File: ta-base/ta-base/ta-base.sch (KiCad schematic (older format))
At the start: 15 parts, among them J1 PinSocket_16_base, J2 PinSocket_4_base, J3 PinSocket_5_base, J4 PinSocket_4_base, J5 PinSocket_5_base, J6 PinSocket_16_base, P1 Gnd_Screws, P2 Gnd_standoffs, SW1 SW_SPDT, SW2 SW_SPDT, U1 BSB008NE2LXXUMA1, U2 burn_wire

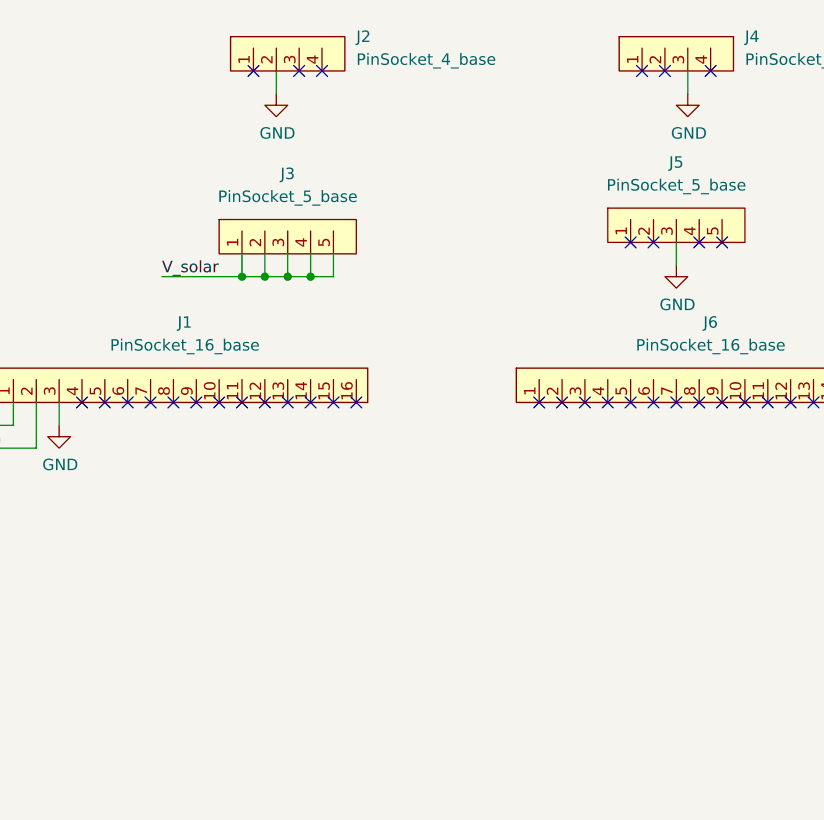
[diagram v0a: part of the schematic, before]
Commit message: finalized place and route
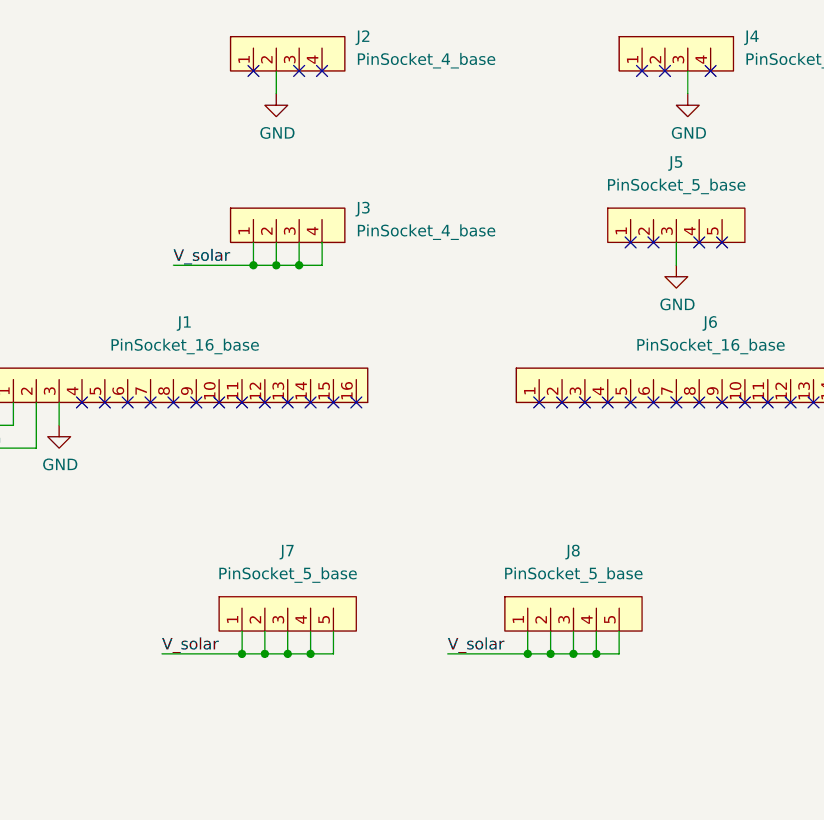
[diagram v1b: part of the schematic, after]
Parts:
- removed J3: PinSocket_5_base, symbol ta-base:PinSocket_5_base
- added J3: PinSocket_4_base, ta-base:PinSocket_1x4_TartanArtibeus_base_cpy, symbol ta-base:PinSocket_4_base
- added J7, J8: PinSocket_5_base, ta-base:solar_internal, symbol ta-base:PinSocket_5_base
- J4: footprint (none) -> ta-base:PinSocket_1x4_TartanArtibeus_base_cpy
- J5: footprint (none) -> ta-base:PinSocket_1x5_right_TartanArtibeus_base_cpy
- J6: footprint (none) -> ta-base:PinSocket_1x16_TartanArtibeus_base_cpy
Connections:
- net V_solar: now also J3.1, J3.2, J3.3, J3.4, J7.1, J7.2, J7.3, J7.4, J7.5, J8.1, J8.2, J8.3, J8.4, J8.5
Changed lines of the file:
@@
 F 0 "J4" H 10000 2100 50  0000 L CNN
 F 1 "PinSocket_4_base" H 10000 2000 50  0000 L CNN
-F 2 "" H 9650 1950 50  0001 C CNN
+F 2 "ta-base:PinSocket_1x4_TartanArtibeus_base_cpy" H 9650 1950 50  0001 C CNN
 F 3 "" H 9650 1950 50  0001 C CNN
 	1    9700 1950
-	1    0    0    -1
-$EndComp
-$Comp
-L ta-base:PinSocket_5_base J3
-U 1 1 60FD2C19
-P 8000 2750
-F 0 "J3" H 8000 3100 50  0000 C CNN
-F 1 "PinSocket_5_base" H 8000 3000 50  0000 C CNN
-F 2 "" H 7900 2750 50  0001 C CNN
-F 3 "" H 7900 2750 50  0001 C CNN
-	1    8000 2750
 	1    0    0    -1
 $EndComp
@@
 F 0 "J5" H 9700 3050 50  0000 C CNN
 F 1 "PinSocket_5_base" H 9700 2950 50  0000 C CNN
-F 2 "" H 9600 2700 50  0001 C CNN
+F 2 "ta-base:PinSocket_1x5_right_TartanArtibeus_base_cpy" H 9600 2700 50  0001 C CNN
 F 3 "" H 9600 2700 50  0001 C CNN
 	1    9700 2700
@@
 F 0 "J6" H 9850 3750 50  0000 C CNN
 F 1 "PinSocket_16_base" H 9850 3650 50  0000 C CNN
-F 2 "" H 9400 3400 50  0001 C CNN
+F 2 "ta-base:PinSocket_1x16_TartanArtibeus_base_cpy" H 9400 3400 50  0001 C CNN
 F 3 "" H 9400 3400 50  0001 C CNN
 	1    9800 3400
@@
 $EndComp
 Wire Wire Line
-	7800 2750 7800 2850
-Wire Wire Line
-	7800 2850 7900 2850
-Wire Wire Line
-	8200 2850 8200 2750
-Wire Wire Line
-	8100 2750 8100 2850
-Connection ~ 8100 2850
-Wire Wire Line
-	8100 2850 8200 2850
-Wire Wire Line
-	8000 2750 8000 2850
-Connection ~ 8000 2850
-Wire Wire Line
-	8000 2850 8100 2850
-Wire Wire Line
-	7900 2750 7900 2850
-Connection ~ 7900 2850
-Wire Wire Line
-	7900 2850 8000 2850
-Wire Wire Line
-	7800 2850 7450 2850
-Connection ~ 7800 2850
-Text Label 7450 2850 0    50   ~ 0
+	7850 2700 7850 2800
+Wire Wire Line
+	7850 2800 7950 2800
+Wire Wire Line
+	8150 2700 8150 2800
+Wire Wire Line
+	8050 2700 8050 2800
+Connection ~ 8050 2800
+Wire Wire Line
+	8050 2800 8150 2800
+Wire Wire Line
+	7950 2700 7950 2800
+Connection ~ 7950 2800
+Wire Wire Line
+	7950 2800 8050 2800
+Wire Wire Line
+	7850 2800 7500 2800
+Connection ~ 7850 2800
+Text Label 7500 2800 0    50   ~ 0
 V_solar
 Wire Wire Line
@@
 Wire Wire Line
 	4000 5950 4150 5950
+$Comp
+L ta-base:PinSocket_4_base J3
+U 1 1 60FB8139
+P 8000 2700
+F 0 "J3" H 8300 2850 50  0000 L CNN
+F 1 "PinSocket_4_base" H 8300 2750 50  0000 L CNN
+F 2 "ta-base:PinSocket_1x4_TartanArtibeus_base_cpy" H 7950 2700 50  0001 C CNN
+F 3 "" H 7950 2700 50  0001 C CNN
+	1    8000 2700
+	1    0    0    -1
+$EndComp
+Wire Wire Line
+	8700 4500 9050 4500
+Connection ~ 9050 4500
+Wire Wire Line
+	9050 4400 9050 4500
+Text Label 8700 4500 0    50   ~ 0
+V_solar
+Connection ~ 9250 4500
+Wire Wire Line
+	9250 4400 9250 4500
+Wire Wire Line
+	9250 4500 9350 4500
+Wire Wire Line
+	9350 4500 9450 4500
+Connection ~ 9350 4500
+Wire Wire Line
+	9350 4400 9350 4500
+Wire Wire Line
+	9450 4400 9450 4500
+Wire Wire Line
+	9150 4500 9050 4500
+Wire Wire Line
+	9150 4500 9250 4500
+Connection ~ 9150 4500
+Wire Wire Line
+	9150 4400 9150 4500
+$Comp
+L ta-base:PinSocket_5_base J8
+U 1 1 60FF8354
+P 9250 4400
+F 0 "J8" H 9250 4750 50  0000 C CNN
+F 1 "PinSocket_5_base" H 9250 4650 50  0000 C CNN
+F 2 "ta-base:solar_internal" H 9150 4400 50  0001 C CNN
+F 3 "" H 9150 4400 50  0001 C CNN
+	1    9250 4400
+	1    0    0    -1
+$EndComp
+Wire Wire Line
+	7450 4500 7800 4500
+Connection ~ 7800 4500
+Wire Wire Line
+	7800 4400 7800 4500
+Text Label 7450 4500 0    50   ~ 0
+V_solar
+Connection ~ 8000 4500
+Wire Wire Line
+	8000 4400 8000 4500
+Wire Wire Line
+	8000 4500 8100 4500
+Wire Wire Line
+	8100 4500 8200 4500
+Connection ~ 8100 4500
+Wire Wire Line
+	8100 4400 8100 4500
+Wire Wire Line
+	8200 4400 8200 4500
+Wire Wire Line
+	7900 4500 7800 4500
+Wire Wire Line
+	7900 4500 8000 4500
+Connection ~ 7900 4500
+Wire Wire Line
+	7900 4400 7900 4500
+$Comp
+L ta-base:PinSocket_5_base J7
+U 1 1 60FE4BFB
+P 8000 4400
+F 0 "J7" H 8000 4750 50  0000 C CNN
+F 1 "PinSocket_5_base" H 8000 4650 50  0000 C CNN
+F 2 "ta-base:solar_internal" H 7900 4400 50  0001 C CNN
+F 3 "" H 7900 4400 50  0001 C CNN
+	1    8000 4400
+	1    0    0    -1
+$EndComp
 $EndSCHEMATC
